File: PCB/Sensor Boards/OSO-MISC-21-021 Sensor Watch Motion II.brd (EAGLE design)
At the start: 14.4 x 7 mm, 8 parts, among them U2 LIS2DW12TR

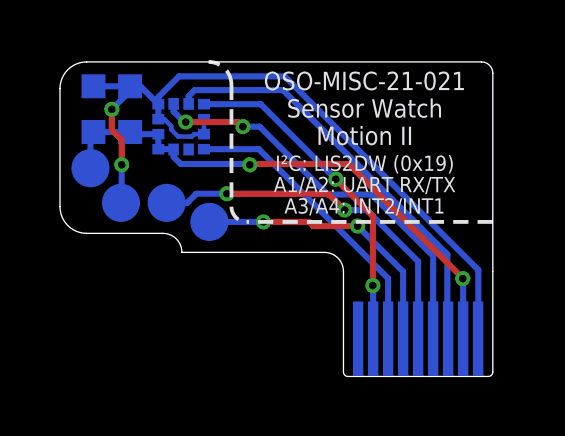
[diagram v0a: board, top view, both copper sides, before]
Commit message: tweaks to the next pair of sensor boards
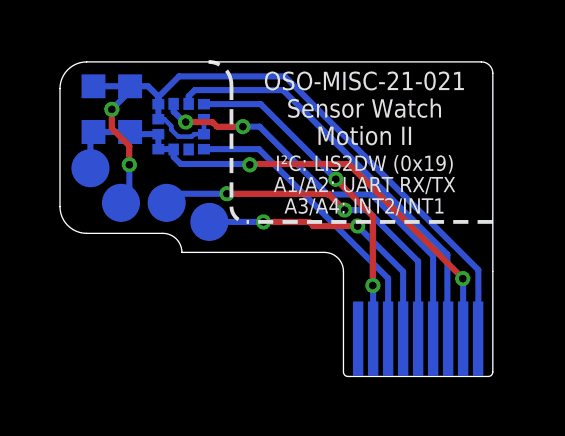
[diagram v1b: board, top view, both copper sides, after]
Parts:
- C1: value 10µF -> 0.1uF
- C2: value 0.1uF -> 10uF
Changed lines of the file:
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@@
 <drawing>
 <settings>
-<setting alwaysvectorfont="no"/>
+<setting alwaysvectorfont="yes"/>
 <setting keepoldvectorfont="yes"/>
 <setting verticaltext="up"/>
 </settings>
-<grid distance="0.01" unitdist="inch" unit="inch" style="lines" multiple="1" display="no" altdistance="0.0005" altunitdist="inch" altunit="inch"/>
+<grid distance="0.01" unitdist="inch" unit="inch" style="lines" multiple="1" display="no" altdistance="0.001" altunitdist="inch" altunit="inch"/>
 <layers>
 <layer number="1" name="Top" color="4" fill="1" visible="yes" active="yes"/>
@@
 </class>
 </classes>
-<designrules name="oshpark-2layer">
+<designrules name="oshpark-2layer *">
 <description language="en">&lt;b&gt;OSH Park Design Rules&lt;/b&gt;
 &lt;p&gt;
@@
 <param name="mlMinCreamFrame" value="0mil"/>
 <param name="mlMaxCreamFrame" value="0mil"/>
-<param name="mlViaStopLimit" value="0mil"/>
+<param name="mlViaStopLimit" value="10mil"/>
 <param name="srRoundness" value="0"/>
 <param name="srMinRoundness" value="0mil"/>
@@
 <elements>
 <element name="U$3" library="FH19C-9S-0.5SH" package="FH19C9S05SH10-FFC" value="FH19C-9S-0.5SH_10-FFC" x="0" y="-2.794" smashed="yes"/>
-<element name="C2" library="microbuilder" package="_0603MP" value="0.1uF" x="-10.8204" y="2.6162" smashed="yes" rot="MR90">
+<element name="C2" library="microbuilder" package="_0603MP" value="10uF" x="-10.8204" y="2.6162" smashed="yes" rot="MR90">
 <attribute name="NAME" x="-12.3698" y="2.6035" size="0.508" layer="26" font="vector" ratio="18" rot="MR90" align="center"/>
 <attribute name="VALUE" x="-11.7729" y="1.6637" size="0.508" layer="28" font="vector" ratio="18" rot="MR90" align="center"/>
 </element>
-<element name="C1" library="microbuilder" package="_0603MP" value="10µF" x="-9.6012" y="2.6162" smashed="yes" rot="MR270">
+<element name="C1" library="microbuilder" package="_0603MP" value="0.1uF" x="-9.6012" y="2.6162" smashed="yes" rot="MR270">
 <attribute name="NAME" x="-9.5758" y="4.8006" size="0.508" layer="26" font="vector" ratio="18" rot="MR180" align="center"/>
 <attribute name="VALUE" x="-8.6487" y="3.5687" size="0.508" layer="28" font="vector" ratio="18" rot="MR270" align="center"/>
@@
 <wire x1="-7.7978" y1="2.1844" x2="-8.1494" y2="2.536" width="0.2032" layer="16"/>
 <via x="-7.747" y="2.1844" extent="1-16" drill="0.254"/>
-<wire x1="-5.9944" y1="2.1844" x2="-7.747" y2="2.1844" width="0.2032" layer="1"/>
-<wire x1="-5.9944" y1="2.1844" x2="-5.842" y2="2.032" width="0.2032" layer="1"/>
+<wire x1="-6.858" y1="2.1844" x2="-7.747" y2="2.1844" width="0.2032" layer="1"/>
+<wire x1="-6.7056" y1="2.032" x2="-6.858" y2="2.1844" width="0.2032" layer="1"/>
+<wire x1="-6.7056" y1="2.032" x2="-5.842" y2="2.032" width="0.2032" layer="1"/>
 <via x="-5.842" y="2.032" extent="1-16" drill="0.254"/>
 <wire x1="-5.2832" y1="2.032" x2="-5.842" y2="2.032" width="0.2032" layer="16"/>
@@
 <wire x1="-2.9939" y1="-0.2032" x2="-6.3754" y2="-0.2032" width="0.2032" layer="1"/>
 <via x="-6.3754" y="-0.2032" extent="1-16" drill="0.254"/>
-<wire x1="-8.382" y1="-0.508" x2="-7.6962" y2="-0.508" width="0.2032" layer="16"/>
-<wire x1="-7.3914" y1="-0.2032" x2="-7.6962" y2="-0.508" width="0.2032" layer="16"/>
-<wire x1="-7.3914" y1="-0.2032" x2="-6.3754" y2="-0.2032" width="0.2032" layer="16"/>
+<wire x1="-6.3754" y1="-0.2032" x2="-8.0772" y2="-0.2032" width="0.2032" layer="16"/>
+<wire x1="-8.382" y1="-0.508" x2="-8.0772" y2="-0.2032" width="0.2032" layer="16"/>
 </signal>
 <signal name="A1_RX">
@@
 <wire x1="-8.6594" y1="2.782" x2="-8.6594" y2="3.0183875" width="0.2032" layer="16"/>
 <wire x1="-8.6594" y1="3.0183875" x2="-7.9693875" y2="3.7084" width="0.2032" layer="16"/>
-<wire x1="-8.6594" y1="2.782" x2="-9.2556" y2="3.3782" width="0.2032" layer="16"/>
-<wire x1="-9.2556" y1="3.3782" x2="-9.6012" y2="3.3782" width="0.2032" layer="16"/>
+<wire x1="-8.6594" y1="2.782" x2="-8.6594" y2="3.036" width="0.2032" layer="16"/>
+<wire x1="-8.6594" y1="3.036" x2="-9.0016" y2="3.3782" width="0.2032" layer="16"/>
+<wire x1="-9.0016" y1="3.3782" x2="-9.6012" y2="3.3782" width="0.2032" layer="16"/>
 <wire x1="-8.6594" y1="2.282" x2="-8.6594" y2="2.782" width="0.2032" layer="16"/>
 <wire x1="-9.6012" y1="3.3782" x2="-9.6012" y2="3.2194" width="0.2032" layer="16"/>
 <wire x1="-9.6012" y1="3.2194" x2="-10.2108" y2="2.6098" width="0.2032" layer="16"/>
 <via x="-10.2108" y="2.6098" extent="1-16" drill="0.254"/>
-<wire x1="-10.2108" y1="2.6098" x2="-10.2108" y2="1.924" width="0.2032" layer="1"/>
-<wire x1="-9.8806" y1="1.5938" x2="-10.2108" y2="1.924" width="0.2032" layer="1"/>
-<wire x1="-9.8806" y1="1.5938" x2="-9.8806" y2="0.762" width="0.2032" layer="1"/>
-<via x="-9.8806" y="0.762" extent="1-16" drill="0.254"/>
-<wire x1="-9.8806" y1="0.762" x2="-9.8806" y2="-0.4826" width="0.2032" layer="16"/>
-<wire x1="-9.8806" y1="-0.4826" x2="-9.906" y2="-0.508" width="0.2032" layer="16"/>
+<wire x1="-9.6266" y1="1.3906" x2="-10.2108" y2="1.9748" width="0.2032" layer="1"/>
+<wire x1="-10.2108" y1="1.9748" x2="-10.2108" y2="2.6098" width="0.2032" layer="1"/>
+<wire x1="-9.6266" y1="1.3906" x2="-9.6266" y2="0.762" width="0.2032" layer="1"/>
+<via x="-9.6266" y="0.762" extent="1-16" drill="0.254"/>
+<wire x1="-9.6266" y1="0.762" x2="-9.6266" y2="-0.2286" width="0.2032" layer="16"/>
+<wire x1="-9.6266" y1="-0.2286" x2="-9.906" y2="-0.508" width="0.2032" layer="16"/>
 <wire x1="-8.2308" y1="1.9349" x2="-8.2308" y2="2.0516875" width="0.1524" layer="16"/>
 <wire x1="-8.6594" y1="2.282" x2="-8.4611125" y2="2.282" width="0.1524" layer="16"/>
